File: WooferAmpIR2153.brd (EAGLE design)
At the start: 142.2 x 47.3 mm, 71 parts

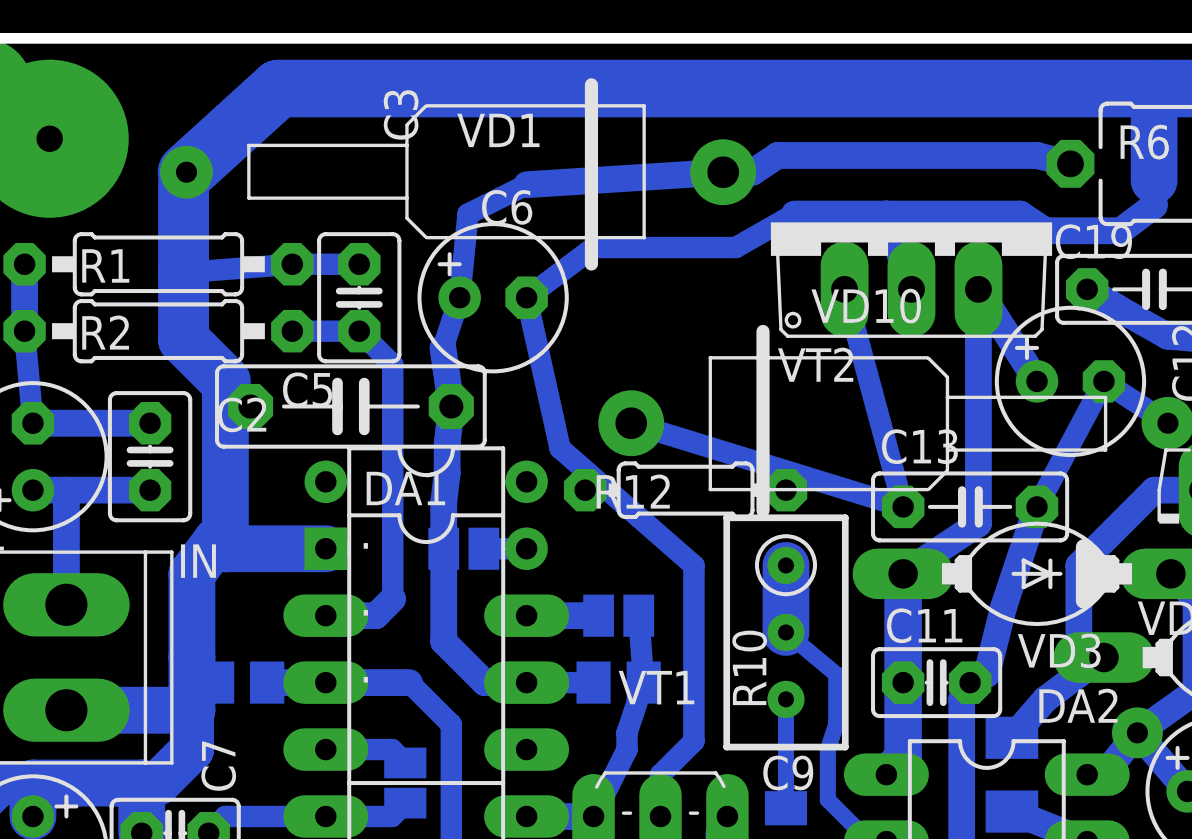
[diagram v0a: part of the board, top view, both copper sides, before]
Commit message: r3
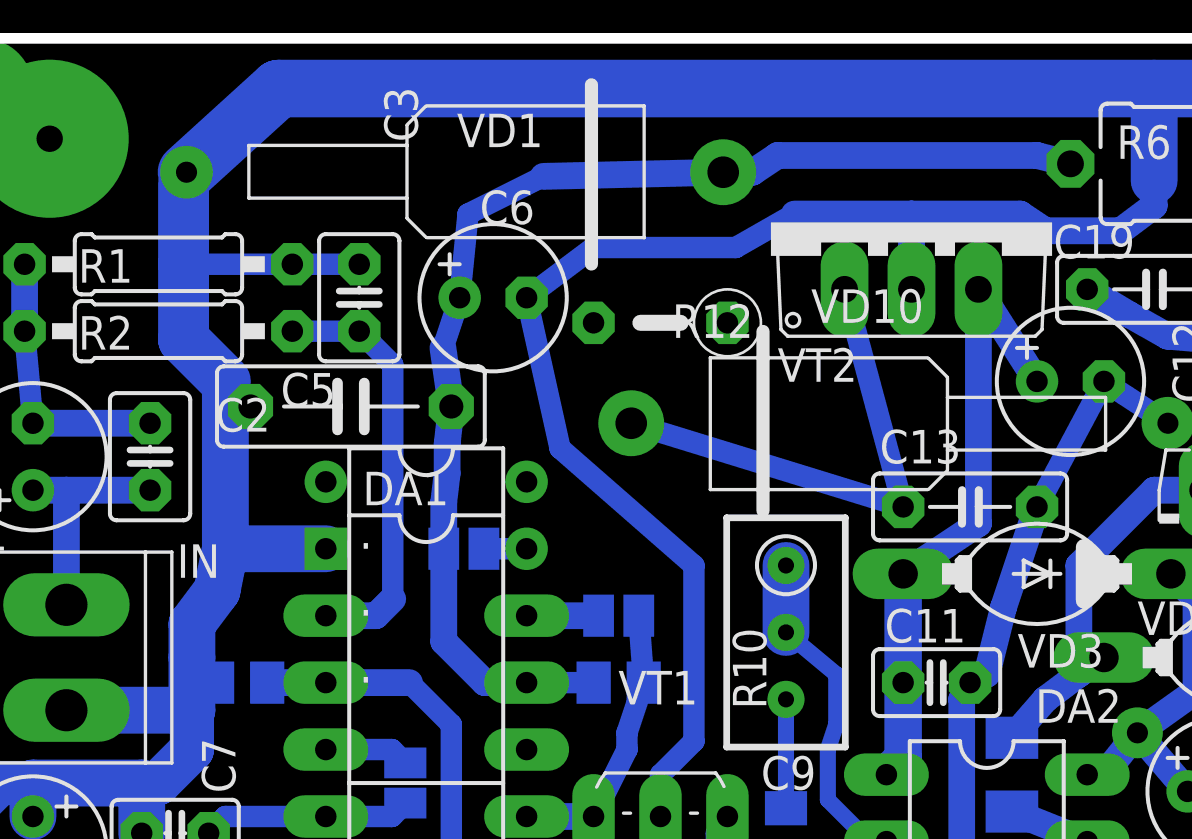
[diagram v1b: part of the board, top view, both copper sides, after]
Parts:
- R12: device resistor:0204/7 -> resistor:0207/5V
- moved R12 6.42 mm to (27.0, 34.9), turned to 180 degrees
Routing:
- net GND: track 386.4 -> 385.5 mm
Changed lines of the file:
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@@
 <?xml version="1.0" encoding="utf-8"?>
 <!DOCTYPE eagle SYSTEM "eagle.dtd">
-<eagle version="6.3">
+<eagle version="6.4">
 <drawing>
 <settings>
@@
 <board>
 <plain>
-<dimension x1="0" y1="-2.54" x2="140.97" y2="-1.27" x3="70.485" y3="-6.985" layer="20" dtype="horizontal"/>
+<dimension x1="0" y1="-2.54" x2="140.97" y2="-1.27" x3="70.485" y3="-6.985" textsize="3.5" layer="20" dtype="horizontal"/>
 <wire x1="-0.635" y1="45.72" x2="141.605" y2="45.72" width="0.4064" layer="20"/>
 <wire x1="141.605" y1="45.72" x2="141.605" y2="-1.5875" width="0.4064" layer="20"/>
 <wire x1="141.605" y1="-1.5875" x2="-0.635" y2="-1.5875" width="0.4064" layer="20"/>
 <wire x1="-0.635" y1="-1.5875" x2="-0.635" y2="45.72" width="0.4064" layer="20"/>
-<dimension x1="144.145" y1="45.72" x2="144.145" y2="0" x3="149.225" y3="22.86" layer="20" dtype="vertical"/>
-<dimension x1="-3.175" y1="45.72" x2="-2.54" y2="-1.5875" x3="-15.875" y3="22.06625" layer="20" dtype="vertical"/>
-<dimension x1="-0.635" y1="-12.7" x2="141.605" y2="-10.4775" x3="70.485" y3="-17.145" layer="20" dtype="horizontal"/>
-<dimension x1="171.45" y1="22.225" x2="-21.2725" y2="45.72" x3="-27.305" y3="33.9725" layer="47" dtype="vertical"/>
-<dimension x1="49.8475" y1="47.3075" x2="113.03" y2="53.0225" x3="81.43875" y3="-26.67" layer="47" dtype="horizontal"/>
+<dimension x1="144.145" y1="45.72" x2="144.145" y2="0" x3="149.225" y3="22.86" textsize="3.5" layer="20" dtype="vertical"/>
+<dimension x1="-3.175" y1="45.72" x2="-2.54" y2="-1.5875" x3="-15.875" y3="22.06625" textsize="3.5" layer="20" dtype="vertical"/>
+<dimension x1="-0.635" y1="-12.7" x2="141.605" y2="-10.4775" x3="70.485" y3="-17.145" textsize="3.5" layer="20" dtype="horizontal"/>
+<dimension x1="171.45" y1="22.225" x2="-21.2725" y2="45.72" x3="-27.305" y3="33.9725" textsize="3.5" layer="47" dtype="vertical"/>
+<dimension x1="49.8475" y1="47.3075" x2="113.03" y2="53.0225" x3="81.43875" y3="-26.67" textsize="3.5" layer="47" dtype="horizontal"/>
 </plain>
 <attributes>
@@
 <attribute name="VALUE" x="31.4325" y="31.115" size="1.27" layer="27" ratio="10"/>
 </element>
-<element name="R12" library="resistor" package="0204/7" value="15k" x="27.94" y="28.575" smashed="yes">
-<attribute name="NAME" x="24.41575" y="27.8765" size="1.27" layer="25" ratio="10"/>
-<attribute name="VALUE" x="28.37815" y="27.94" size="1.27" layer="27" ratio="10"/>
+<element name="R12" library="resistor" package="0207/5V" value="15k" x="26.9875" y="34.925" smashed="yes" rot="R180">
+<attribute name="NAME" x="30.51175625" y="35.6235" size="1.27" layer="25" ratio="10" rot="R180"/>
+<attribute name="VALUE" x="26.549353125" y="35.560003125" size="1.27" layer="27" ratio="10" rot="R180"/>
 </element>
 <element name="VD4" library="diode" package="ZDIO-10" value="15v" x="38.735" y="50.8" smashed="yes">
@@
 <wire x1="10.4775" y1="32.7025" x2="8.89" y2="34.29" width="1.9304" layer="16"/>
 <wire x1="12.495" y1="43.815" x2="9.0025" y2="40.64" width="2.1844" layer="16"/>
-<wire x1="8.89" y1="34.29" x2="8.89" y2="36.83" width="1.9304" layer="16"/>
-<wire x1="8.89" y1="36.83" x2="8.89" y2="40.21" width="1.9304" layer="16"/>
+<wire x1="8.89" y1="34.29" x2="8.89" y2="37.1475" width="1.9304" layer="16"/>
+<wire x1="8.89" y1="37.1475" x2="8.89" y2="40.21" width="1.9304" layer="16"/>
 <wire x1="8.89" y1="40.21" x2="9.0025" y2="40.64" width="1.778" layer="16"/>
-<wire x1="10.16" y1="26.67" x2="9.2075" y2="25.4" width="1.778" layer="16"/>
-<wire x1="9.2075" y1="25.4" x2="9.2075" y2="22.225" width="1.778" layer="16"/>
+<wire x1="10.16" y1="24.765" x2="9.2075" y2="23.495" width="1.778" layer="16"/>
+<wire x1="9.2075" y1="23.495" x2="9.2075" y2="22.225" width="1.778" layer="16"/>
 <wire x1="9.2075" y1="22.225" x2="9.2075" y2="20.225" width="1.778" layer="16"/>
 <wire x1="9.2075" y1="20.225" x2="4.445" y2="20.225" width="1.778" layer="16"/>
@@
 <wire x1="0.9525" y1="10.6375" x2="2.065" y2="9.525" width="1.6764" layer="16"/>
 <wire x1="45.72" y1="43.815" x2="45.72" y2="40.3225" width="1.778" layer="16"/>
-<wire x1="35.56" y1="39.0525" x2="32.0675" y2="39.0525" width="1.016" layer="16"/>
-<wire x1="36.5125" y1="36.195" x2="35.56" y2="39.0525" width="1.016" layer="16"/>
-<wire x1="35.56" y1="39.0525" x2="40.64" y2="39.0525" width="1.016" layer="16"/>
+<wire x1="36.5125" y1="39.0525" x2="32.0675" y2="39.0525" width="1.016" layer="16"/>
+<wire x1="36.5125" y1="36.195" x2="36.5125" y2="39.0525" width="1.016" layer="16"/>
+<wire x1="36.5125" y1="39.0525" x2="40.64" y2="39.0525" width="1.016" layer="16"/>
 <wire x1="40.64" y1="39.0525" x2="41.5925" y2="38.4175" width="1.016" layer="16"/>
 <wire x1="41.5925" y1="38.4175" x2="44.45" y2="38.4175" width="1.016" layer="16"/>
@@
 <contactref element="C22" pad="2"/>
 <contactref element="DA1" pad="2"/>
-<wire x1="10.16" y1="26.67" x2="10.4775" y2="26.3525" width="1.778" layer="16"/>
+<wire x1="10.16" y1="24.765" x2="10.4775" y2="26.3525" width="1.778" layer="16"/>
 <wire x1="10.4775" y1="26.3525" x2="10.4775" y2="32.0675" width="1.778" layer="16"/>
 <wire x1="10.4775" y1="32.0675" x2="10.4775" y2="32.7025" width="1.778" layer="16"/>
@@
 <wire x1="10.795" y1="31.75" x2="10.4775" y2="32.0675" width="0.8128" layer="16"/>
 <wire x1="13.0175" y1="37.1475" x2="15.5575" y2="37.1475" width="0.8128" layer="16"/>
-<wire x1="13.0175" y1="37.1475" x2="8.89" y2="36.83" width="0.8128" layer="16"/>
+<wire x1="13.0175" y1="37.1475" x2="8.89" y2="37.1475" width="0.8128" layer="16"/>
 <wire x1="26.9875" y1="16.1925" x2="26.9875" y2="17.78" width="0.8128" layer="16"/>
 <wire x1="26.9875" y1="17.78" x2="28.2575" y2="19.05" width="0.8128" layer="16"/>
@@
 <wire x1="28.2575" y1="25.7175" x2="23.1775" y2="30.1625" width="0.8128" layer="16"/>
 <wire x1="23.1775" y1="30.1625" x2="21.9075" y2="35.8775" width="0.8128" layer="16"/>
-<wire x1="23.1775" y1="30.1625" x2="24.13" y2="28.575" width="0" layer="19" extent="16-16"/>
+<wire x1="29.845" y1="37.7825" x2="29.5275" y2="34.925" width="0" layer="19" extent="16-16"/>
 </signal>
 <signal name="N$4">
@@
 <wire x1="36.195" y1="27.94" x2="25.8775" y2="31.115" width="0.8128" layer="16"/>
 <wire x1="33.9725" y1="36.195" x2="36.195" y2="27.94" width="0.8128" layer="16"/>
-<wire x1="36.195" y1="27.94" x2="31.75" y2="28.575" width="0" layer="19" extent="1-1"/>
+<wire x1="25.8775" y1="31.115" x2="24.4475" y2="34.925" width="0" layer="19" extent="1-1"/>
 </signal>
 <signal name="V15+">
@@
 <wire x1="31.4325" y1="41.275" x2="41.275" y2="41.275" width="1.016" layer="16"/>
 <wire x1="41.275" y1="41.275" x2="42.545" y2="40.9575" width="1.016" layer="16"/>
-<wire x1="29.3675" y1="40.64" x2="21.9075" y2="40.165" width="1.016" layer="16"/>
+<wire x1="29.3675" y1="40.64" x2="22.5425" y2="40.4825" width="1.016" layer="16"/>
 <wire x1="18.7325" y1="33.9725" x2="19.05" y2="31.75" width="1.016" layer="16"/>
 <contactref element="DA1" pad="11"/>
@@
 <wire x1="18.7325" y1="33.9725" x2="19.3675" y2="35.8775" width="0.8128" layer="16"/>
 <wire x1="19.3675" y1="35.8775" x2="19.685" y2="39.0525" width="0.8128" layer="16"/>
-<wire x1="19.685" y1="39.0525" x2="21.9075" y2="40.165" width="0.8128" layer="16"/>
+<wire x1="19.685" y1="39.0525" x2="22.5425" y2="40.4825" width="0.8128" layer="16"/>
 </signal>
 <signal name="N$35">

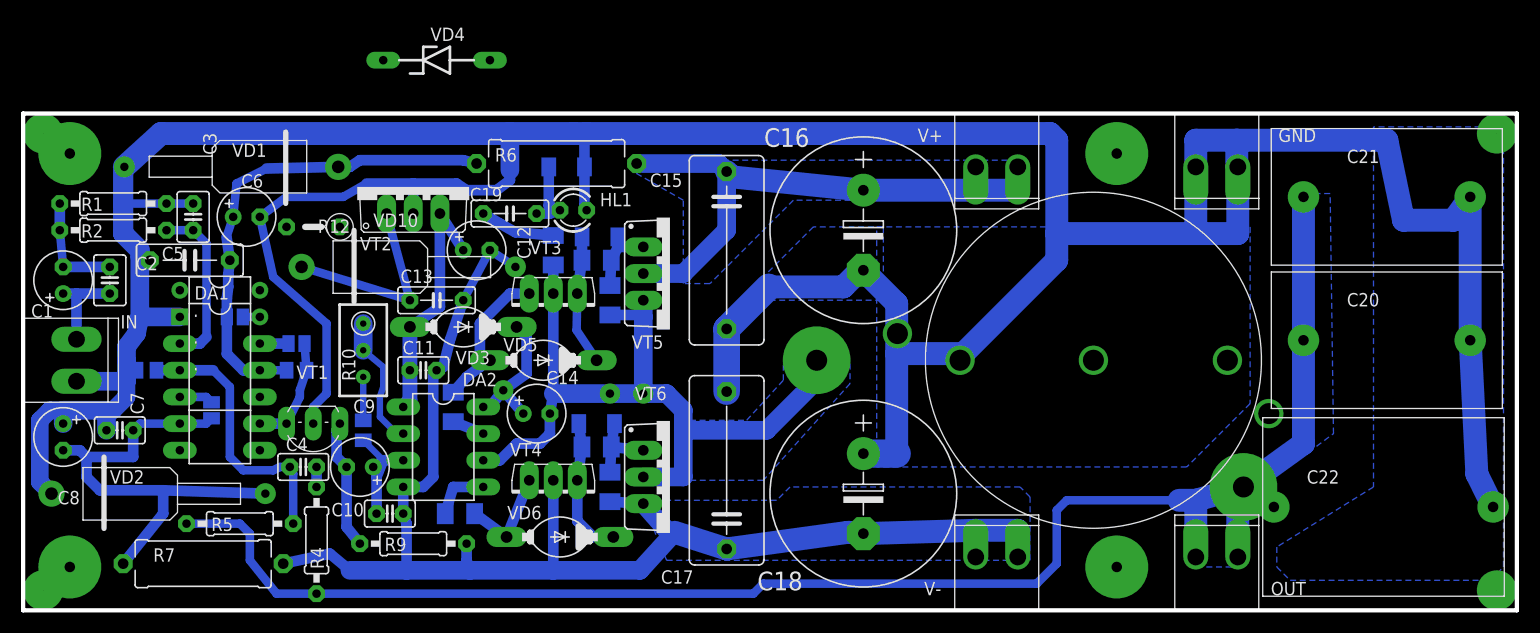
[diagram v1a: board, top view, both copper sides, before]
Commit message: h2
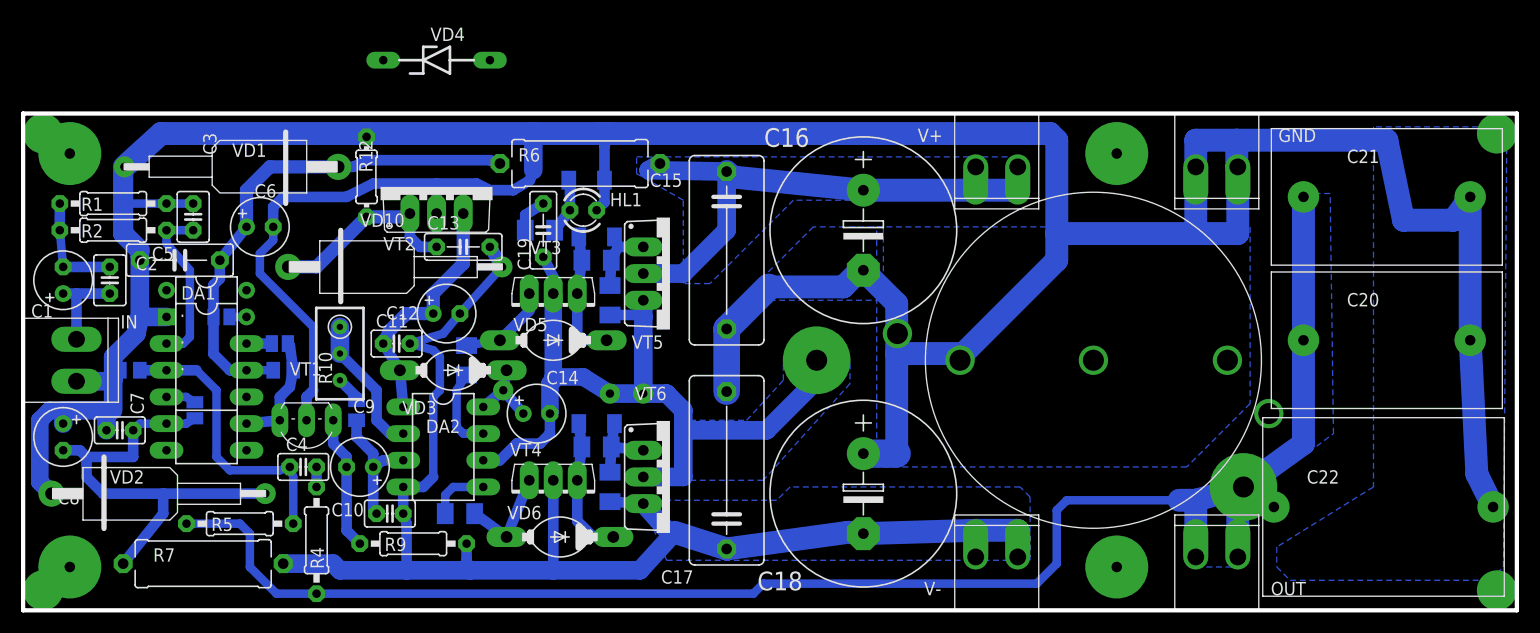
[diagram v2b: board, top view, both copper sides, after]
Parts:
- R12: device resistor:0207/5V -> resistor:0204/7
- moved R12 6.96 mm to (32.1, 39.7), turned to 270 degrees
- moved C12 6.68 mm to (39.7, 26.7)
- moved C13 5.68 mm to (41.3, 33.0)
- moved R13 4.62 mm to (41.6, 22.2)
- moved VD3 4.24 mm to (40.3, 21.3)
- moved C11 3.59 mm to (34.9, 23.8)
- moved C19 3.55 mm to (48.9, 34.6), turned to 90 degrees
- moved VD9 2.29 mm to (53.0, 39.4)
- moved R19 2.29 mm to (48.6, 34.6), turned to 0 degrees
- moved R10 2.25 mm to (29.5, 22.9)
- moved R6 2.22 mm to (52.4, 41.0)
- moved VT2 2.22 mm to (38.7, 38.7)
- moved VD5 2.13 mm to (49.8, 24.1)
- moved R11 2.01 mm to (31.1, 17.5)
- moved R3 1.59 mm to (9.53, 21.3)
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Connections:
- net N$10: now also R19.1; no longer C19.2
- net N$9: now also C19.2, R19.2; no longer C19.1, R19.1
- net NL: now also C19.1; no longer R19.2
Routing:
- net VB: track 13.2 -> 7.34 mm
- net N$17: track 14.6 -> 8.82 mm
- net N$12: track 3.08 -> 8.04 mm
- net N$9: track 7.16 -> 3.49 mm
- net V-: track 133.6 -> 136.2 mm
- net VC+: track 46.1 -> 48.3 mm
- net VC-: track 45.2 -> 43.4 mm
- net N$10: track 7.12 -> 5.30 mm
- net N$4: track 10.9 -> 12.7 mm
- net N$6: track 4.13 -> 2.57 mm
- net NL: track 75.4 -> 77.0 mm
- net C-: track 26.1 -> 27.5 mm
- net V15+: track 24.3 -> 23.4 mm
- net N$1: track 12.7 -> 13.4 mm
- net GND: track 385.5 -> 386.0 mm, vias 0 -> 2
